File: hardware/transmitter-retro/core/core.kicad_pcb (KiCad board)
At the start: 2 copper layers, 100 x 90 mm, 64 parts, among them J1 Input, J2 Output, J3 Power, J4 Expansion, U1 556, U10 74LS163, U11 TLC7524CN, U12 74LS245, U13 74LS153, U14 74LS04, U15 74LS74, U16 74LS74, U18 74LS32, U19 74LS08, U2 74LS163, U21 LM339, U6 74LS153, U7 74LS273, U8 74LS165, U9 74LS163, Y1 4Mz

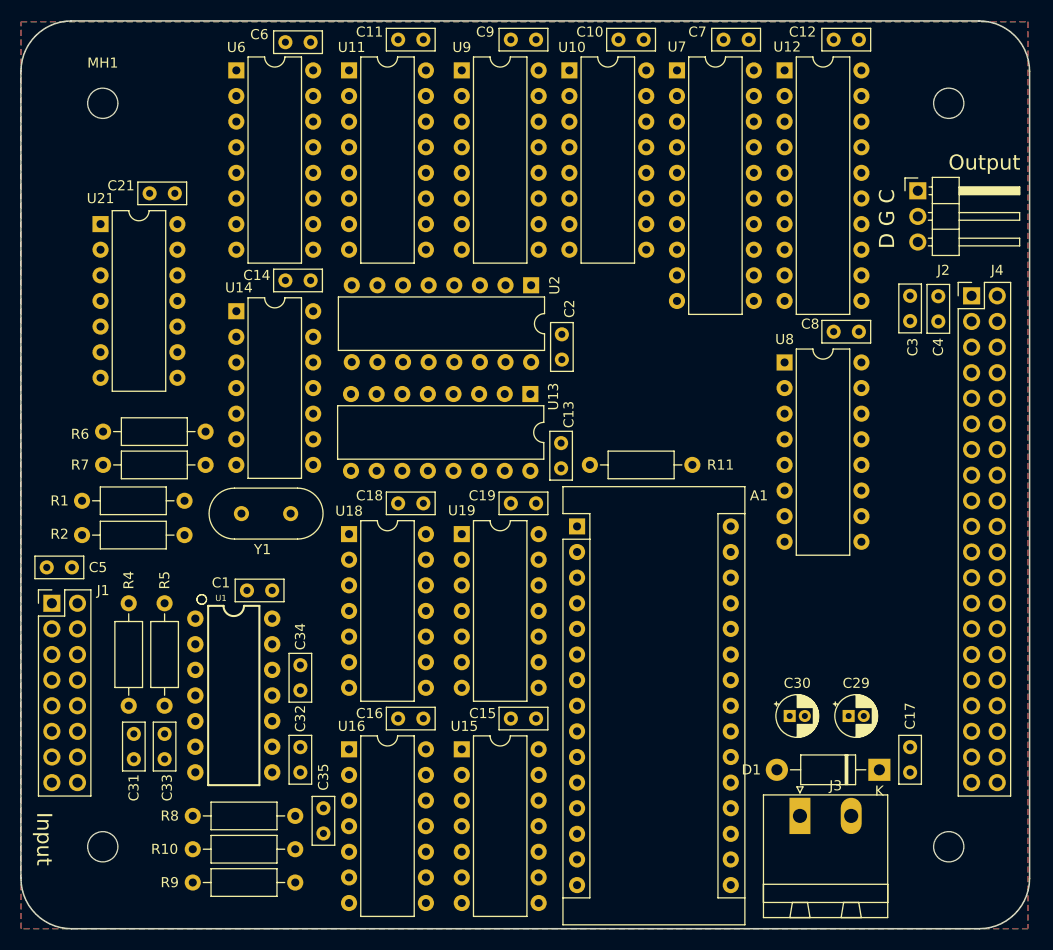
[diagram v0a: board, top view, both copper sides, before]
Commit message: Update part numbers Swap out input connector footprint Placement tweaks
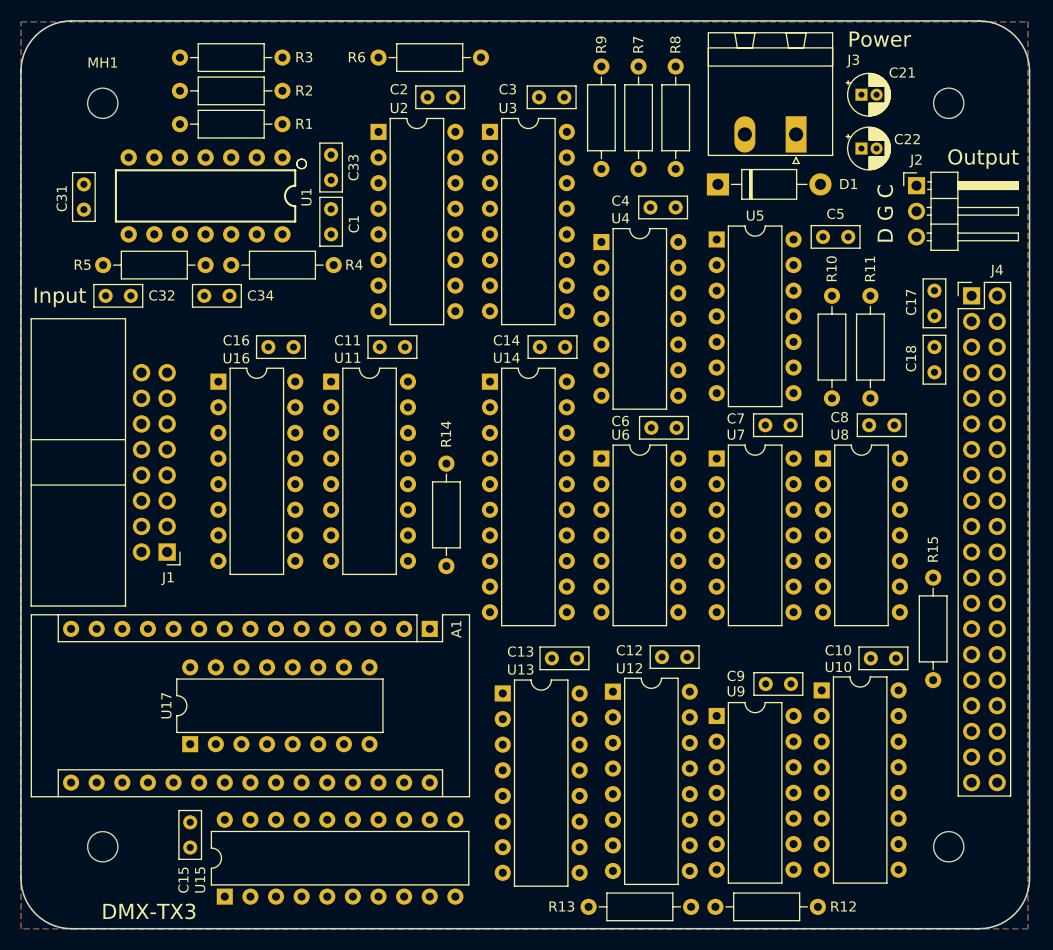
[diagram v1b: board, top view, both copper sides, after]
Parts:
- removed C19: .01uF, Capacitor_THT:C_Rect_L4.6mm_W2.0mm_P2.50mm_MKS02_FKP02
- removed C29, C30: CP1, Capacitor_THT:CP_Radial_D4.0mm_P1.50mm
- removed C35: .001uF, Capacitor_THT:C_Rect_L4.6mm_W2.0mm_P2.50mm_MKS02_FKP02
- removed U18: 74LS32, Package_DIP:DIP-14_W7.62mm
- removed U19: 74LS08, Package_DIP:DIP-14_W7.62mm
- removed U21: LM339, Package_DIP:DIP-14_W7.62mm
- removed Y1: 4Mz, Crystal:Crystal_HC49-U_Vertical
- added C22: CP1, Capacitor_THT:CP_Radial_D4.0mm_P1.50mm, F.Cu at (170.4, 61.3)
- added R12: 10k, Resistor_THT:R_Axial_DIN0207_L6.3mm_D2.5mm_P10.16mm_Horizontal, F.Cu at (166.1, 136.5)
- added R13: 10k, Resistor_THT:R_Axial_DIN0207_L6.3mm_D2.5mm_P10.16mm_Horizontal, F.Cu at (143.4, 136.5)
- added R14: 10k, Resistor_THT:R_Axial_DIN0207_L6.3mm_D2.5mm_P10.16mm_Horizontal, F.Cu at (129.3, 92.6)
- added R15: 10k, Resistor_THT:R_Axial_DIN0207_L6.3mm_D2.5mm_P10.16mm_Horizontal, F.Cu at (177.5, 114.0)
- added R3: 1M, Resistor_THT:R_Axial_DIN0207_L6.3mm_D2.5mm_P10.16mm_Horizontal, F.Cu at (102.9, 52.3)
- added U17: ULN2003A, Package_DIP:DIP-16_W7.62mm, F.Cu at (103.9, 120.4)
- added U3: 74LS163, Package_DIP:DIP-16_W7.62mm, F.Cu at (133.6, 59.7)
- added U4: 74LS74, Package_DIP:DIP-14_W7.62mm, F.Cu at (144.7, 70.6)
- added U5: 74LS74, Package_DIP:DIP-14_W7.62mm, F.Cu at (156.1, 70.4)
- C21: value .01uF -> CP1; footprint Capacitor_THT:C_Rect_L4.6mm_W2.0mm_P2.50mm_MKS02_FKP02 -> Capacitor_THT:CP_Radial_D4.0mm_P1.50mm
- J1: footprint Connector_PinHeader_2.54mm:PinHeader_2x08_P2.54mm_Vertical -> Connector_IDC:IDC-Header_2x08_P2.54mm_Horizontal
- R10, R9: value 100k -> 10k
- R6, R7: value 2.2k -> 10k
- U10: value 74LS163 -> 74LS165
- U11: value TLC7524CN -> 74LS151
- U12: value 74LS245 -> 74LS163; footprint Package_DIP:DIP-20_W7.62mm -> Package_DIP:DIP-16_W7.62mm
- U13: value 74LS153 -> 74LS163
- U14: value 74LS04 -> 74LS373; footprint Package_DIP:DIP-14_W7.62mm -> Package_DIP:DIP-20_W7.62mm
- U15: value 74LS74 -> TLC7524CN; footprint Package_DIP:DIP-14_W7.62mm -> Package_DIP:DIP-20_W7.62mm
- U16: value 74LS74 -> LM339; footprint Package_DIP:DIP-14_W7.62mm -> Package_DIP:DIP-16_W7.62mm
- U2: value 74LS163 -> 74LS151
- U6: value 74LS153 -> 74LS08; footprint Package_DIP:DIP-16_W7.62mm -> Package_DIP:DIP-14_W7.62mm
- U7: value 74LS273 -> 74LS32; footprint Package_DIP:DIP-20_W7.62mm -> Package_DIP:DIP-14_W7.62mm
- U8: value 74LS165 -> 74LS04; footprint Package_DIP:DIP-16_W7.62mm -> Package_DIP:DIP-14_W7.62mm
- U9: value 74LS163 -> 74LS02; footprint Package_DIP:DIP-16_W7.62mm -> Package_DIP:DIP-14_W7.62mm
- moved R9 86.4 mm to (144.7, 53.2), turned to 270 degrees
- moved C5 83.6 mm to (166.6, 70.1)
- moved R8 83.3 mm to (152.0, 53.2), turned to 270 degrees
- moved R10 76.4 mm to (167.5, 75.9), turned to 270 degrees
- moved U9 68.8 mm to (156.1, 117.6)
- moved C21 68.8 mm to (170.4, 56.0), turned to 0 degrees
- moved C9 68.7 mm to (163.4, 114.4)
- moved J3 67.6 mm to (164.0, 59.9), turned to 180 degrees
- moved U10 66.4 mm to (166.5, 115.1)
- moved C10 66.2 mm to (173.9, 111.9)
- moved U12 63.9 mm to (145.8, 115.2)
- moved C12 63.5 mm to (153.2, 111.8)
- moved D1 60.2 mm to (156.2, 64.9), turned to 0 degrees
- moved C33 59.7 mm to (117.9, 62.0)
- moved R7 58.3 mm to (148.3, 53.2), turned to 270 degrees
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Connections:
- A1 pad 1: /SAMPLE_LATCH -> /~SAMPLE_OVERRIDE
- A1 pad 10: /SHIFT_TRANSMIT -> /~SHIFT_ENABLE
- A1 pad 11: /CLK_RX -> /SHIFT_TRANSMIT
- A1 pad 12: /monitor/DATA_RX_IN -> /DATA_RX
- A1 pad 13: /CLK_FAST -> /CLK_RX
- A1 pad 14: /CLK_SLOW -> /CLK_FAST
- A1 pad 15: /~SAMPLE_ASSERT -> /CLK_SLOW
- A1 pad 5: /~SAMPLE_RESET -> /SAMPLE_LATCH
- A1 pad 6: /SAMPLE_SEL0 -> /~SAMPLE_RESET
- A1 pad 7: /SAMPLE_SEL1 -> /SAMPLE_SEL0
- A1 pad 8: /~SHIFT_LOAD -> /SAMPLE_SEL1
- A1 pad 9: /SHIFT_DISABLE -> /~SHIFT_LOAD
- J1 pad 3: /monitor/DATA_RX_IN -> /shift/~CLK_OUT
- J1 pad 5: /CLK_RX -> /shift/~DATA_OUT
- J2 pad 3: /monitor/DATA_RX_IN -> /DATA_RX
- J4 pad 10: /~SAMPLE_RESET -> /SAMPLE_LATCH
- J4 pad 12: /SAMPLE_SEL0 -> /~SAMPLE_RESET
- J4 pad 14: /SAMPLE_SEL1 -> /SAMPLE_SEL0
- J4 pad 16: /~SHIFT_LOAD -> /SAMPLE_SEL1
- J4 pad 18: /SHIFT_DISABLE -> /~SHIFT_LOAD
- J4 pad 20: /SHIFT_TRANSMIT -> /~SHIFT_ENABLE
- J4 pad 21: /CLK_TX -> /~BUS_ACK
- J4 pad 22: /DATA_FIXED -> /SHIFT_TRANSMIT
- J4 pad 23: /CLK_RX -> /~BUS_REQ
- J4 pad 24: /~FRAME_RESET -> Net-(J4-Pad24)
- J4 pad 25: /CLK_FAST -> /SAMPLE_REF
- J4 pad 26: Net-(J4-Pad26) -> /~FRAME_RESET
- J4 pad 27: /CLK_SLOW -> /CLK_EXT
- J4 pad 28: Net-(J4-Pad28) -> /DATA_RX
- J4 pad 29: Net-(J4-Pad29) -> /CLK_TX
- J4 pad 30: Net-(J4-Pad30) -> /DATA_FIXED
- J4 pad 31: Net-(J4-Pad31) -> /CLK_RX
- J4 pad 32: Net-(J4-Pad32) -> /DATA_SHIFT
- J4 pad 33: Net-(J4-Pad33) -> /CLK_FAST
- J4 pad 34: Net-(J4-Pad34) -> GND
- J4 pad 35: Net-(J4-Pad35) -> /CLK_SLOW
- J4 pad 36: Net-(J4-Pad36) -> GND
- J4 pad 37: GND -> Net-(J4-Pad37)
- J4 pad 39: GND -> /~CLK_EXT_SEL
- J4 pad 6: /~SAMPLE_ASSERT -> /SAMPLE_COUNT
- J4 pad 8: /SAMPLE_LATCH -> /~SAMPLE_OVERRIDE
- R10 pad 1: /clock/~CLK_SLOW_IN -> +5V
- R10 pad 2: GND -> /shift/~CLK_STEP_IN
- R11 pad 2: /shift/~CLK_STEP_IN -> /clock/~CLK_STEP_INA
- R6 pad 1: Net-(R6-Pad1) -> +5V
- R6 pad 2: Net-(R6-Pad2) -> /CLK_EXT
- R7 pad 1: Net-(R7-Pad1) -> +5V
- R7 pad 2: Net-(R6-Pad1) -> /clock/~CLK_SLOW_IN
- R8 pad 1: /clock/~CLK_STEP_INA -> +5V
- R8 pad 2: GND -> /clock/~CLK_FAST_IN
- R9 pad 1: /clock/~CLK_FAST_IN -> +5V
- R9 pad 2: GND -> /~CLK_EXT_SEL
- U1 pad 5: Net-(U1-Pad5) -> /clock/CLK_SLOW
- U1 pad 9: Net-(U1-Pad9) -> /clock/CLK_FAST
- U10 pad 1: /~SAMPLE_RESET -> /~SHIFT_LOAD
- U10 pad 10: Net-(U10-Pad10) -> GND
- U10 pad 11: /sample/DO7 -> /shift/D0
- U10 pad 12: /sample/DO6 -> /shift/D1
- U10 pad 13: /sample/DO5 -> /shift/D2
- U10 pad 14: /sample/DO4 -> /shift/D3
- U10 pad 15: Net-(U10-Pad15) -> /~SHIFT_ENABLE
- U10 pad 2: /clock/CLK_SAMPLE_OUT -> /CLK_TX
- U10 pad 3: GND -> /shift/D4
- U10 pad 4: GND -> /shift/D5
- U10 pad 5: GND -> /shift/D6
- U10 pad 6: GND -> /shift/D7
- U10 pad 7: +5V -> Net-(U10-Pad7)
- U10 pad 9: +5V -> /DATA_SHIFT
- U11 pad 1: +5V -> Net-(U11-Pad1)
- U11 pad 10: /sample/DO1 -> Net-(U11-Pad10)
- U11 pad 11: /sample/DO0 -> Net-(U11-Pad11)
- U11 pad 12: GND -> Net-(U11-Pad12)
- U11 pad 13: /clock/CLK_SAMPLE_OUT -> Net-(U11-Pad13)
- U11 pad 14: +5V -> Net-(U11-Pad14)
- U11 pad 15: Net-(U11-Pad15) -> /SAMPLE_COUNT
- U11 pad 16: Net-(U11-Pad16) -> +5V
- U11 pad 2: GND -> Net-(U11-Pad2)
- U11 pad 3: GND -> Net-(U11-Pad3)
- U11 pad 4: /sample/DO7 -> Net-(U11-Pad4)
- U11 pad 5: /sample/DO6 -> Net-(U11-Pad5)
- U11 pad 6: /sample/DO5 -> Net-(U11-Pad6)
- U11 pad 7: /sample/DO4 -> GND
- U11 pad 8: /sample/DO3 -> GND
- U11 pad 9: /sample/DO2 -> /~SAMPLE_OVERRIDE
- U12 pad 1: +5V -> /~SAMPLE_RESET
- U12 pad 10: GND -> Net-(U12-Pad10)
- U12 pad 11: /sample/D7 -> /sample/DO3
- U12 pad 12: /sample/D6 -> /sample/DO2
- U12 pad 13: /sample/D5 -> /sample/D01
- U12 pad 14: /sample/D4 -> /sample/DO0
- U12 pad 15: /sample/D3 -> Net-(U12-Pad15)
- U12 pad 16: /sample/D2 -> +5V
- U12 pad 2: Net-(U12-Pad2) -> /clock/CLK_SAMPLE_OUT
- U12 pad 3: Net-(U12-Pad3) -> GND
- U12 pad 4: Net-(U12-Pad4) -> GND
- U12 pad 5: Net-(U12-Pad5) -> GND
- U12 pad 6: Net-(U12-Pad6) -> GND
- U12 pad 7: Net-(U12-Pad7) -> Net-(U11-Pad5)
- U12 pad 8: Net-(U12-Pad8) -> GND
- U12 pad 9: Net-(U12-Pad9) -> +5V
- U13 pad 1: GND -> /~SAMPLE_RESET
- U13 pad 10: GND -> Net-(U12-Pad15)
- U13 pad 11: GND -> /sample/DO7
- U13 pad 12: GND -> /sample/DO6
- U13 pad 13: GND -> /sample/DO5
- U13 pad 14: /CLK_SLOW -> /sample/DO4
- U13 pad 15: GND -> Net-(U13-Pad15)
- U13 pad 2: /CLK_FAST -> /clock/CLK_SAMPLE_OUT
- U13 pad 3: Net-(U13-Pad3) -> GND
- U13 pad 4: Net-(U1-Pad5) -> GND
- U13 pad 5: Net-(U1-Pad9) -> GND
- U13 pad 6: Net-(R7-Pad1) -> GND
- U13 pad 7: /clock/CLK_SAMPLE_OUT -> +5V
- U13 pad 9: Net-(U13-Pad9) -> +5V
- U14 pad 1: Net-(R6-Pad2) -> Net-(U14-Pad1)
- U14 pad 10: Net-(U14-Pad10) -> GND
- U14 pad 11: Net-(U10-Pad15) -> /SAMPLE_LATCH
- U14 pad 12: Net-(U14-Pad12) -> /sample/D4
- U14 pad 13: Net-(U14-Pad13) -> /sample/DO4
- U14 pad 14: +5V -> /sample/DO5
- U14 pad 2: Net-(R6-Pad1) -> /sample/D0
- U14 pad 3: Net-(R6-Pad1) -> /sample/DO0
- U14 pad 4: Net-(R7-Pad1) -> /sample/D01
- U14 pad 5: Net-(U14-Pad5) -> /sample/D1
- U14 pad 6: Net-(U14-Pad6) -> /sample/D2
- U14 pad 7: GND -> /sample/DO2
- U14 pad 8: /CLK_RX -> /sample/DO3
- U14 pad 9: /CLK_TX -> /sample/D3
- U15 pad 10: Net-(U14-Pad12) -> /sample/DO1
- U15 pad 11: Net-(U13-Pad3) -> /sample/DO0
- U15 pad 12: /CLK_TX -> GND
- U15 pad 13: Net-(U15-Pad13) -> /clock/CLK_SAMPLE_OUT
- U15 pad 2: Net-(U15-Pad2) -> GND
- U15 pad 3: Net-(U1-Pad9) -> GND
- U15 pad 4: +5V -> /sample/DO7
- U15 pad 5: Net-(U15-Pad5) -> /sample/DO6
- U15 pad 6: Net-(U15-Pad6) -> /sample/DO5
- U15 pad 7: GND -> /sample/DO4
- U15 pad 8: Net-(U15-Pad8) -> /sample/DO3
- U15 pad 9: Net-(U15-Pad9) -> /sample/DO2
- U16 pad 1: Net-(U16-Pad1) -> Net-(U11-Pad3)
- U16 pad 10: Net-(U16-Pad10) -> /SAMPLE_REF
- U16 pad 11: /CLK_TX -> /sample/DIM_2_IN
- U16 pad 12: /clock/~CLK_FAST_IN -> GND
- U16 pad 13: Net-(U16-Pad10) -> Net-(U11-Pad2)
- U16 pad 14: +5V -> Net-(U11-Pad1)
- U16 pad 2: /clock/~CLK_SLOW_IN -> Net-(U11-Pad4)
- U16 pad 3: /CLK_TX -> +5V
- U16 pad 4: Net-(U16-Pad1) -> /SAMPLE_REF
- U16 pad 5: /CLK_SLOW -> /sample/DIM_4_IN
- U16 pad 6: Net-(U16-Pad6) -> /SAMPLE_REF
- U16 pad 7: GND -> /sample/DIM_3_IN
- U16 pad 8: Net-(U16-Pad8) -> /SAMPLE_REF
- U16 pad 9: /CLK_FAST -> /sample/DIM_1_IN
- U2 pad 1: +5V -> /clock/CLK_STEP
- U2 pad 10: +5V -> /CLK_FAST
- U2 pad 11: /CLK_TX -> /CLK_SLOW
- U2 pad 2: /clock/CLK_SAMPLE_OUT -> /clock/CLK_SLOW
- U2 pad 3: GND -> /clock/CLK_FAST
- U2 pad 4: GND -> /CLK_EXT
- U2 pad 5: GND -> /clock/CLK_SAMPLE_OUT
- U2 pad 6: GND -> Net-(U2-Pad6)
- U2 pad 7: +5V -> GND
- U2 pad 9: +5V -> GND
- U6 pad 1: GND -> /DATA_SHIFT
- U6 pad 10: GND -> Net-(U6-Pad10)
- U6 pad 11: GND -> Net-(U5-Pad2)
- U6 pad 12: GND -> /shift/~CLK_STEP_IN
- U6 pad 13: GND -> /clock/~CLK_STEP_INA
- U6 pad 14: /SAMPLE_SEL0 -> +5V
- U6 pad 2: /SAMPLE_SEL1 -> /SHIFT_TRANSMIT
- U6 pad 3: Net-(U21-Pad14) -> Net-(U6-Pad3)
- U6 pad 4: Net-(U21-Pad13) -> /clock/CLK_FAST
- U6 pad 5: Net-(U21-Pad1) -> Net-(U6-Pad5)
- U6 pad 6: Net-(U21-Pad2) -> /clock/CLK_STEP
- U6 pad 7: Net-(U6-Pad7) -> GND
- U6 pad 8: GND -> Net-(U6-Pad8)
- U6 pad 9: Net-(U6-Pad9) -> Net-(U5-Pad13)
- U7 pad 1: +5V -> Net-(U6-Pad3)
- U7 pad 10: GND -> Net-(U5-Pad2)
- U7 pad 11: /SAMPLE_LATCH -> Net-(U6-Pad5)
- U7 pad 12: Net-(U12-Pad6) -> /CLK_TX
- U7 pad 13: /sample/DO4 -> Net-(U5-Pad8)
- U7 pad 14: /sample/DO5 -> +5V
- U7 pad 2: Net-(U12-Pad2) -> /DATA_FIXED
- U7 pad 3: /sample/DO0 -> /DATA_RX
- U7 pad 4: /sample/D01 -> +5V
- U7 pad 5: Net-(U12-Pad3) -> +5V
- U7 pad 6: Net-(U12-Pad4) -> Net-(U7-Pad6)
- U7 pad 7: /sample/DO2 -> GND
- U7 pad 8: /sample/DO3 -> Net-(U5-Pad13)
- U7 pad 9: Net-(U12-Pad5) -> Net-(U5-Pad6)
- U8 pad 1: /~SHIFT_LOAD -> /~BUS_REQ
- U8 pad 10: GND -> Net-(U8-Pad10)
- U8 pad 11: /shift/D0 -> +5V
- U8 pad 12: /shift/D1 -> Net-(U5-Pad10)
- U8 pad 13: /shift/D2 -> Net-(U6-Pad8)
- U8 pad 14: /shift/D3 -> +5V
- U8 pad 2: /CLK_TX -> Net-(U14-Pad1)
- U8 pad 3: /shift/D4 -> Net-(U14-Pad1)
- U8 pad 4: /shift/D5 -> /~BUS_ACK
- U8 pad 5: /shift/D6 -> Net-(U6-Pad5)
- U8 pad 6: /shift/D7 -> Net-(U6-Pad10)
- U8 pad 7: Net-(U8-Pad7) -> GND
- U8 pad 8: GND -> /CLK_RX
- U8 pad 9: Net-(U19-Pad1) -> /CLK_TX
- U9 pad 1: /~SAMPLE_RESET -> Net-(U11-Pad11)
- U9 pad 10: Net-(U14-Pad10) -> Net-(U12-Pad10)
- U9 pad 11: /sample/DO3 -> +5V
- U9 pad 12: /sample/DO2 -> +5V
- U9 pad 13: /sample/D01 -> Net-(U9-Pad13)
- U9 pad 14: /sample/DO0 -> +5V
- U9 pad 2: /clock/CLK_SAMPLE_OUT -> /~SAMPLE_OVERRIDE
- U9 pad 3: GND -> /SAMPLE_SEL0
- U9 pad 4: GND -> Net-(U11-Pad10)
- U9 pad 5: GND -> /~SAMPLE_OVERRIDE
- U9 pad 6: GND -> /SAMPLE_SEL1
- U9 pad 7: Net-(U6-Pad7) -> GND
- U9 pad 8: GND -> Net-(U13-Pad15)
- U9 pad 9: +5V -> Net-(U13-Pad15)
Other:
- board text added: "DMX-TX3"
- board text added: "DMX-TX3, Rev 1.2 Crazy Giraffe Software"
- board text added: "Power"
- board text removed: "DMX-CPCB, Rev 1.2 Crazy Giraffe Software"
